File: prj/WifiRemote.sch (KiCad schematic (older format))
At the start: 68 parts, among them J1 DIP-BLACK-MALE-HEADER-VERT_4P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, J2 DIP-BLACK-MALE-HEADER_6P-2.54_, K1 DIP-SWITCH-TACTILE-SPST-NO_TS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, K2 DIP-SWITCH-TACTILE-SPST-NO_TS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, K3 DIP-SWITCH-TACTILE-SPST-NO_TS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, K4 DIP-SWITCH-TACTILE-SPST-NO_TS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, M1 Mechanical_Mount, M2 Mechanical_Mount, M3 Mechanical_Mount, M4 Mechanical_Mount, Q1 SMD-MOSFET-P-CH-20V-2A-FDN340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, SW1 DIP-TOGGLE-SWITCH-ON-ON_3+2P-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, U1 CONTROLLER-ESP8266, U2 BOOST-MCP1642B-ADJI/MC-MSOP8

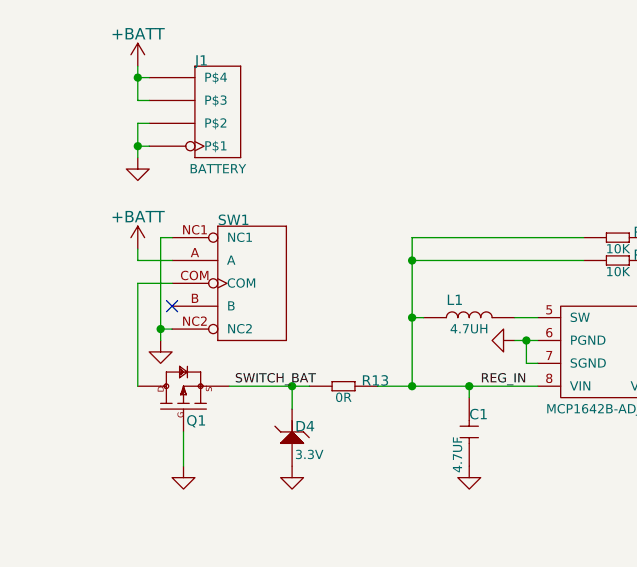
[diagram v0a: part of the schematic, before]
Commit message: Routing has begun
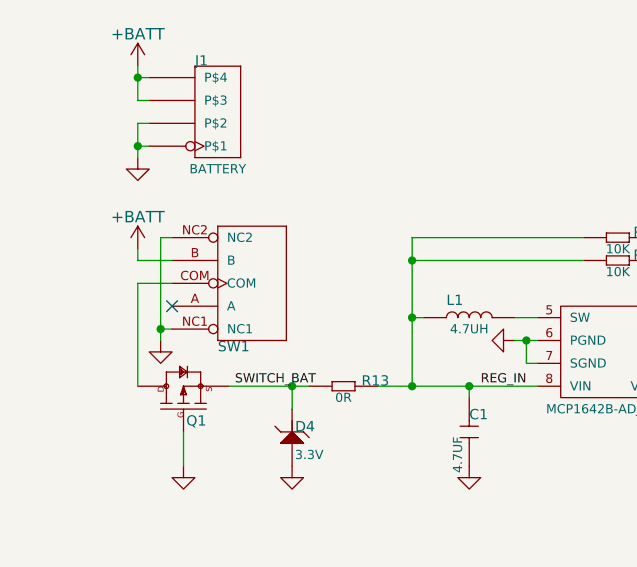
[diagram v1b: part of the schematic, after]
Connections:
- net +BATT: now also SW1.B; no longer SW1.A
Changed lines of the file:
@@
 F 5 "311030008" H 1280 1850 20  0001 C CNN "SKU"
 	1    1250 1700
-	1    0    0    -1
+	1    0    0    1
 $EndComp
 $Comp
